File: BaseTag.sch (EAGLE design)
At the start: 27 parts, among them U1 BQ25504, U3 MSP430FR2512IPW16RSOIC

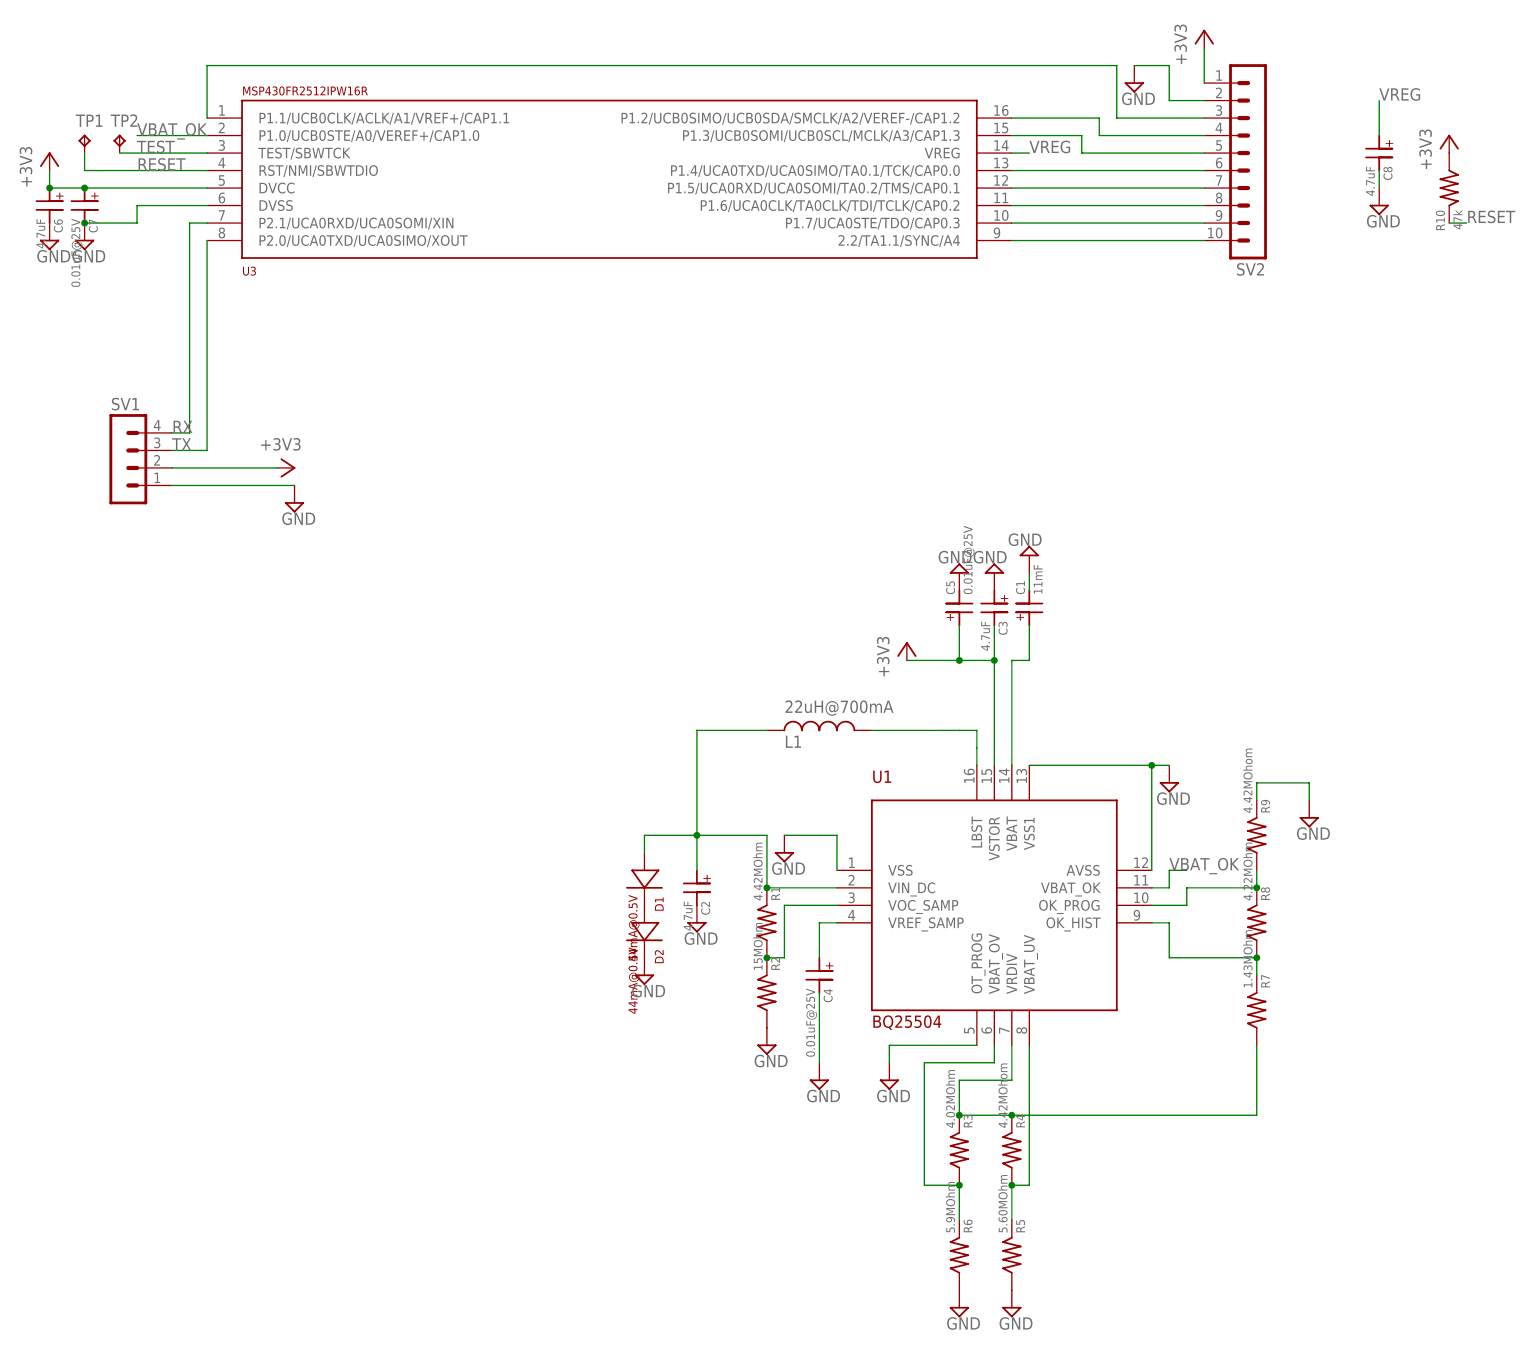
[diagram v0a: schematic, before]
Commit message: alpha layout
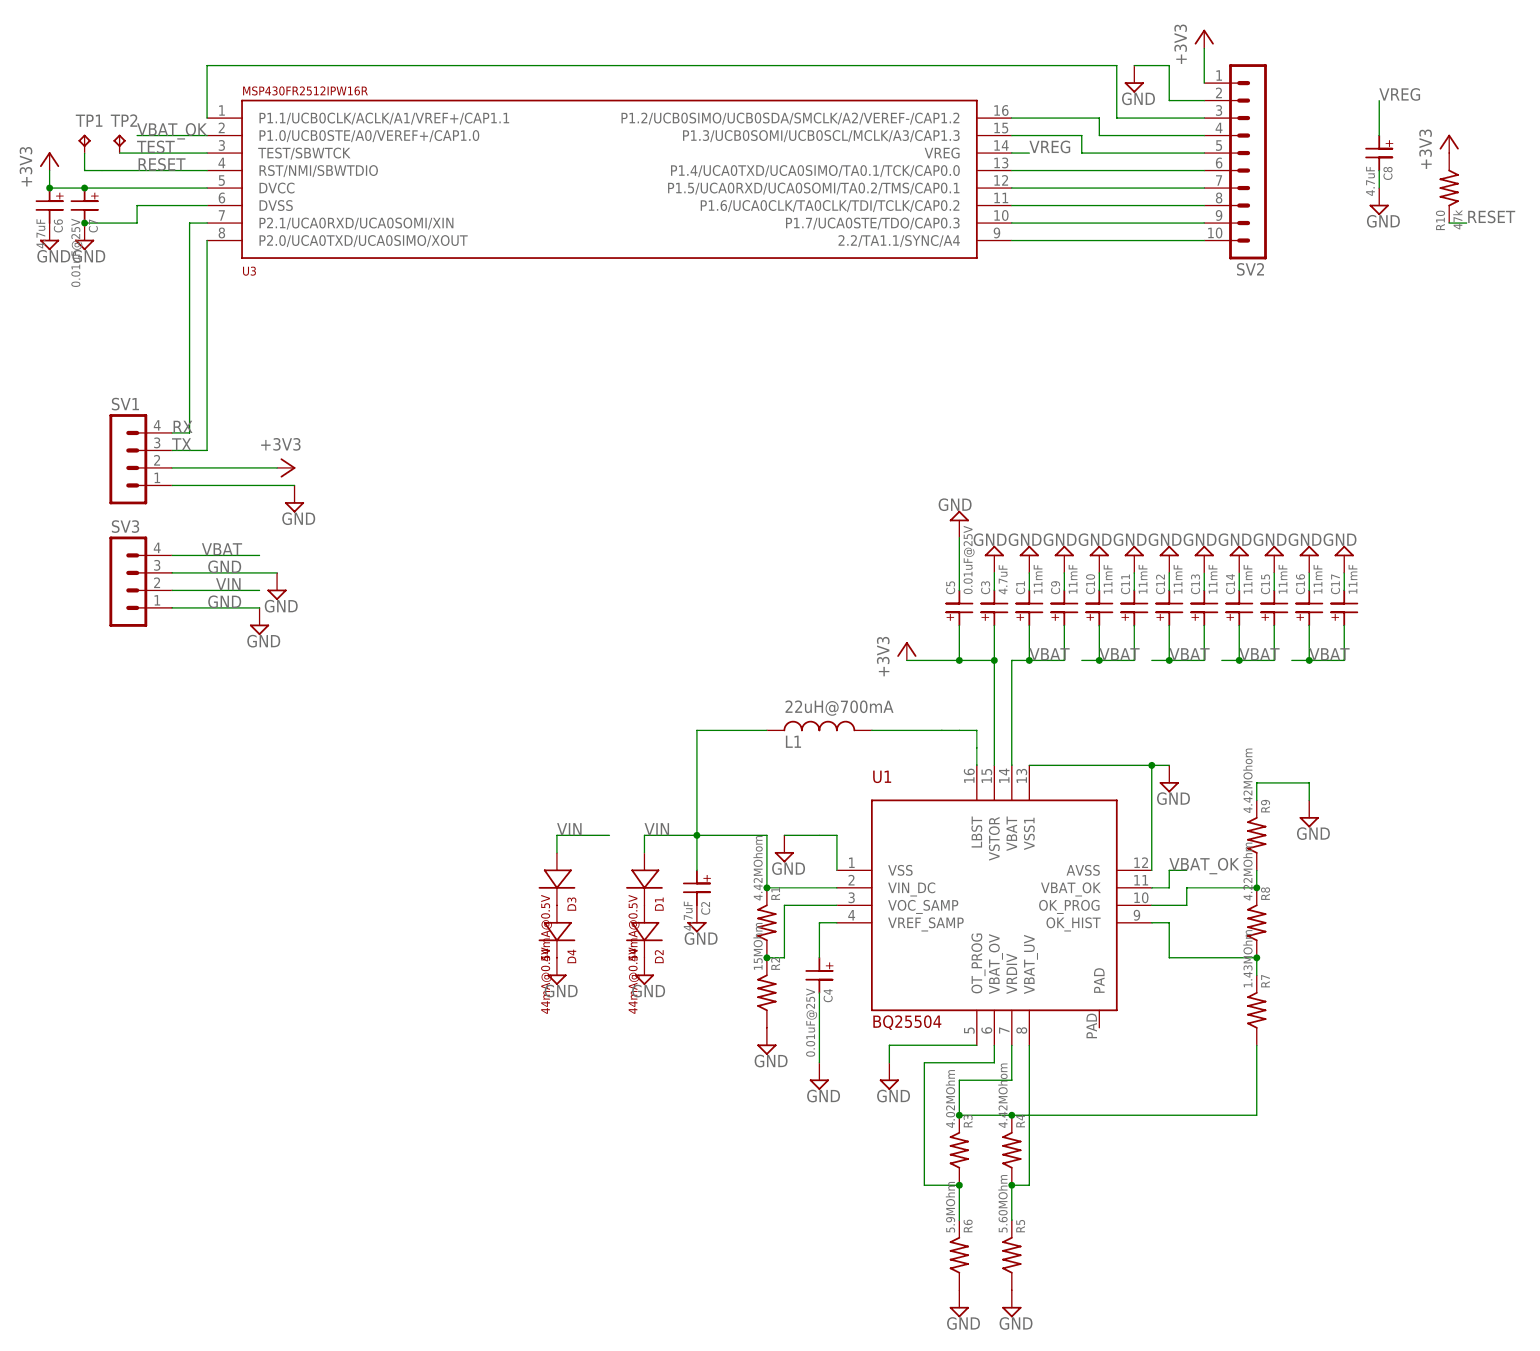
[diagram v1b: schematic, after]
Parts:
- added C10, C11, C12, C13, C14, C15, C16, C17, C9: 11mF, Nelson-RLCD:C
- added D3, D4: 44mA@0.5V, Nelson-IC:SOLAR-CELL
- added SV3: (no value), con-lstb:MA04-1
- C1: device Nelson-RLCD:C11MF1210 -> Nelson-RLCD:C
- R1: value 4.42MOhm -> 4.42MOhom
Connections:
- removed net N$8: C1.+, U1.VBAT
- new net VBAT: C1.+, C10.+, C11.+, C12.+, C13.+, C14.+, C15.+, C16.+, C17.+, C9.+, SV3.4, U1.VBAT
- new net VIN: C2.+, D1.+, D3.+, L1.P$1, R1.P$2, SV3.2, U1.VIN_DC
- net +3V3: now also C3.+; no longer C3.-
- net GND: now also C10.-, C11.-, C12.-, C13.-, C14.-, C15.-, C16.-, C17.-, C3.-, C9.-, D4.-, SV3.1, SV3.3; no longer C3.+
- net N$1: now also D3.-, D4.+; no longer C2.+, D1.+, L1.P$1, R1.P$2, U1.VIN_DC
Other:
- moved on the sheet: C3

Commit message: prep for 1" branch
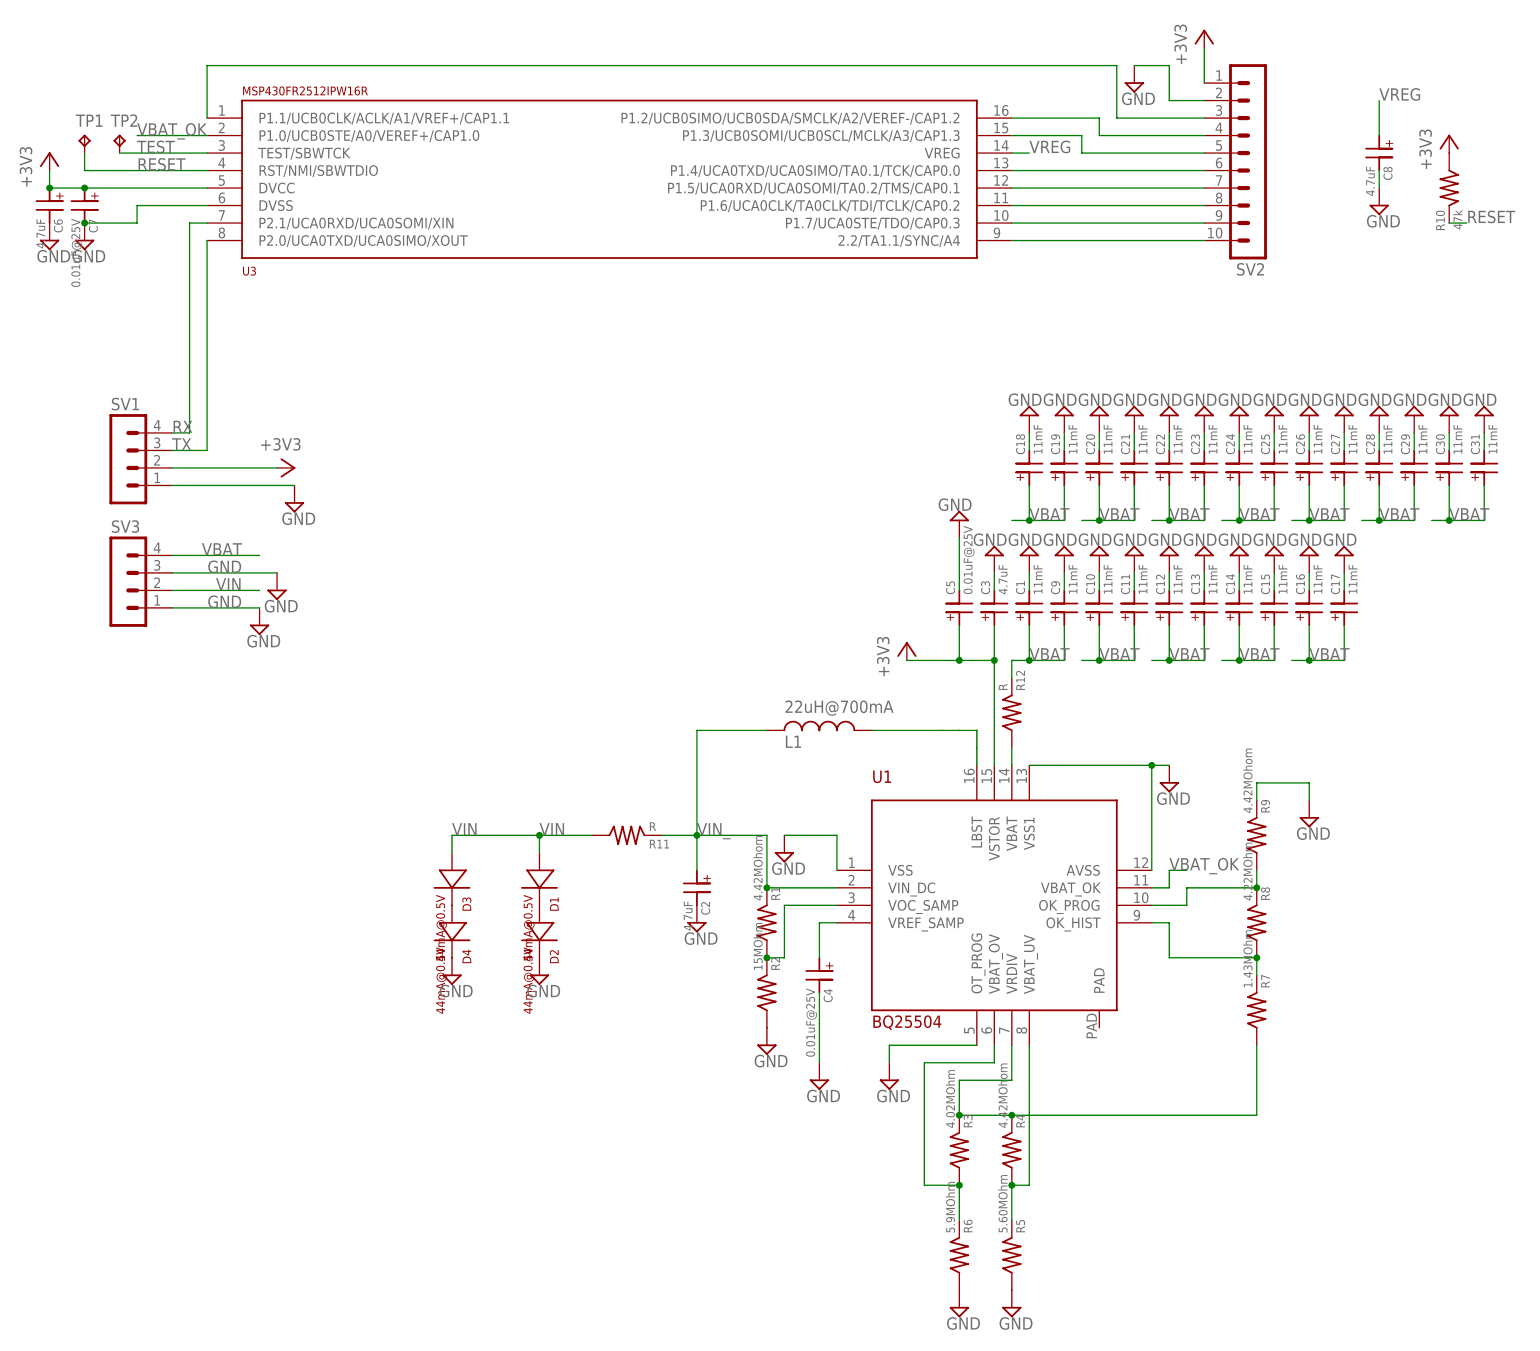
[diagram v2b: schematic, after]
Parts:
- added C18, C19, C20, C21, C22, C23, C24, C25, C26, C27, C28, C29, C30, C31: 11mF, Nelson-RLCD:C
- added R11, R12: R, Nelson-RLCD:R
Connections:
- new net N$8: R12.P$1, U1.VBAT
- new net VIN_: C2.+, L1.P$1, R1.P$2, R11.P$2, U1.VIN_DC
- net GND: now also C18.-, C19.-, C20.-, C21.-, C22.-, C23.-, C24.-, C25.-, C26.-, C27.-, C28.-, C29.-, C30.-, C31.-
- net VBAT: now also C18.+, C19.+, C20.+, C21.+, C22.+, C23.+, C24.+, C25.+, C26.+, C27.+, C28.+, C29.+, C30.+, C31.+, R12.P$2; no longer U1.VBAT
- net VIN: now also R11.P$1; no longer C2.+, L1.P$1, R1.P$2, U1.VIN_DC
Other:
- moved on the sheet: D1, D2, D3, D4
